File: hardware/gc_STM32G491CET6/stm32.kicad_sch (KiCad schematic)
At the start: 22 parts, among them J7 Conn_02x07_Odd_Even, Y301 16MHz

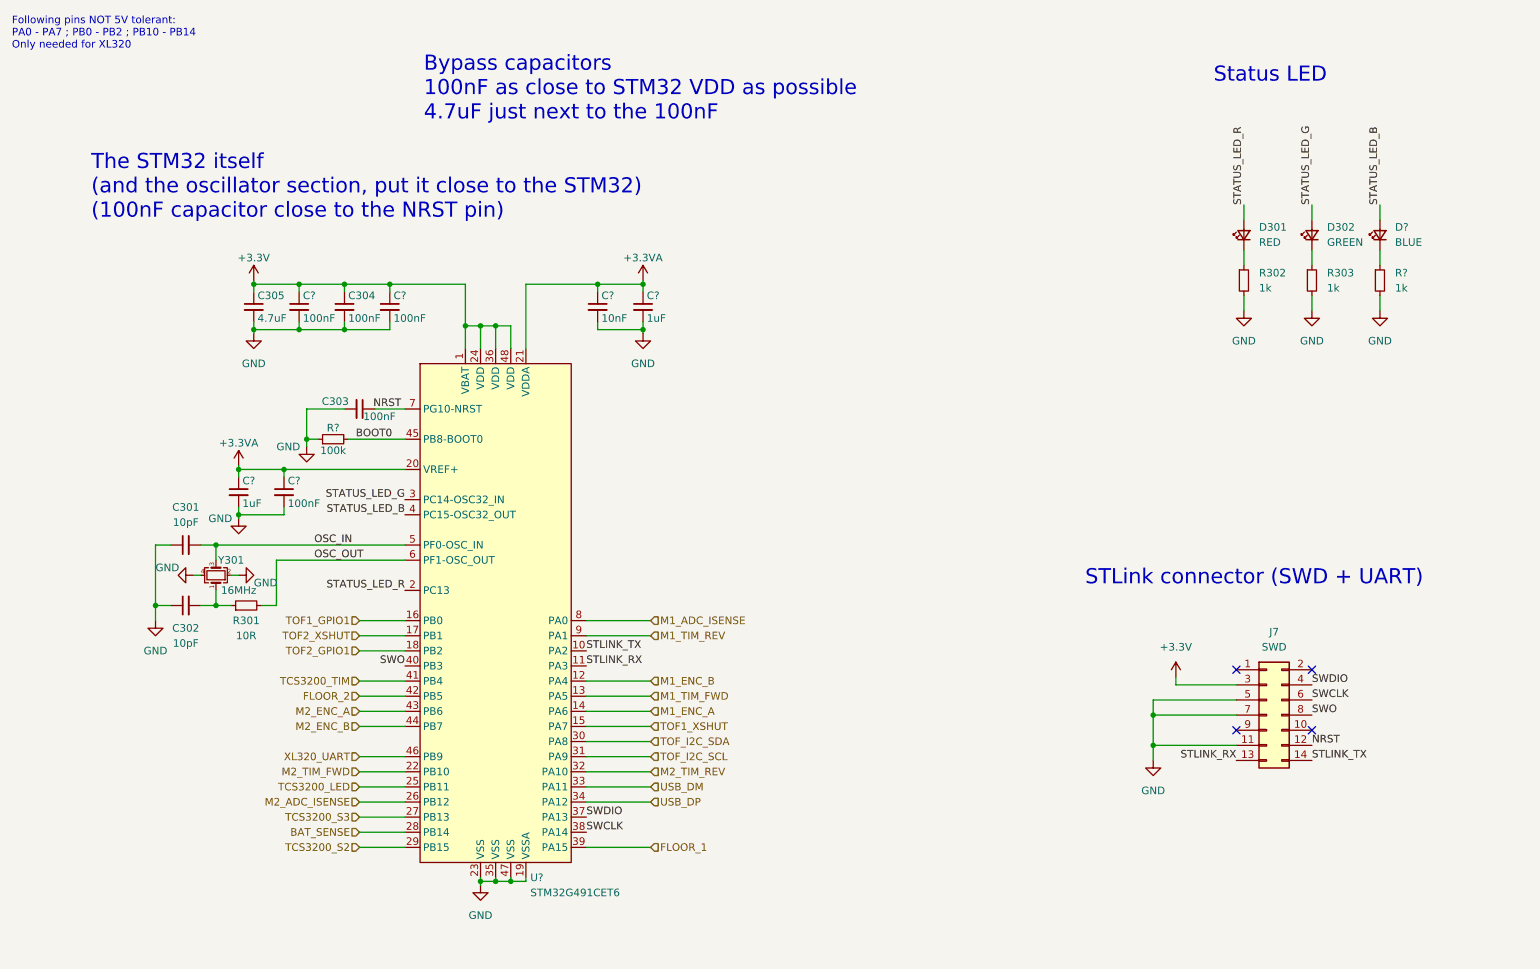
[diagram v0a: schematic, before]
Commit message: Schematics + rough placement
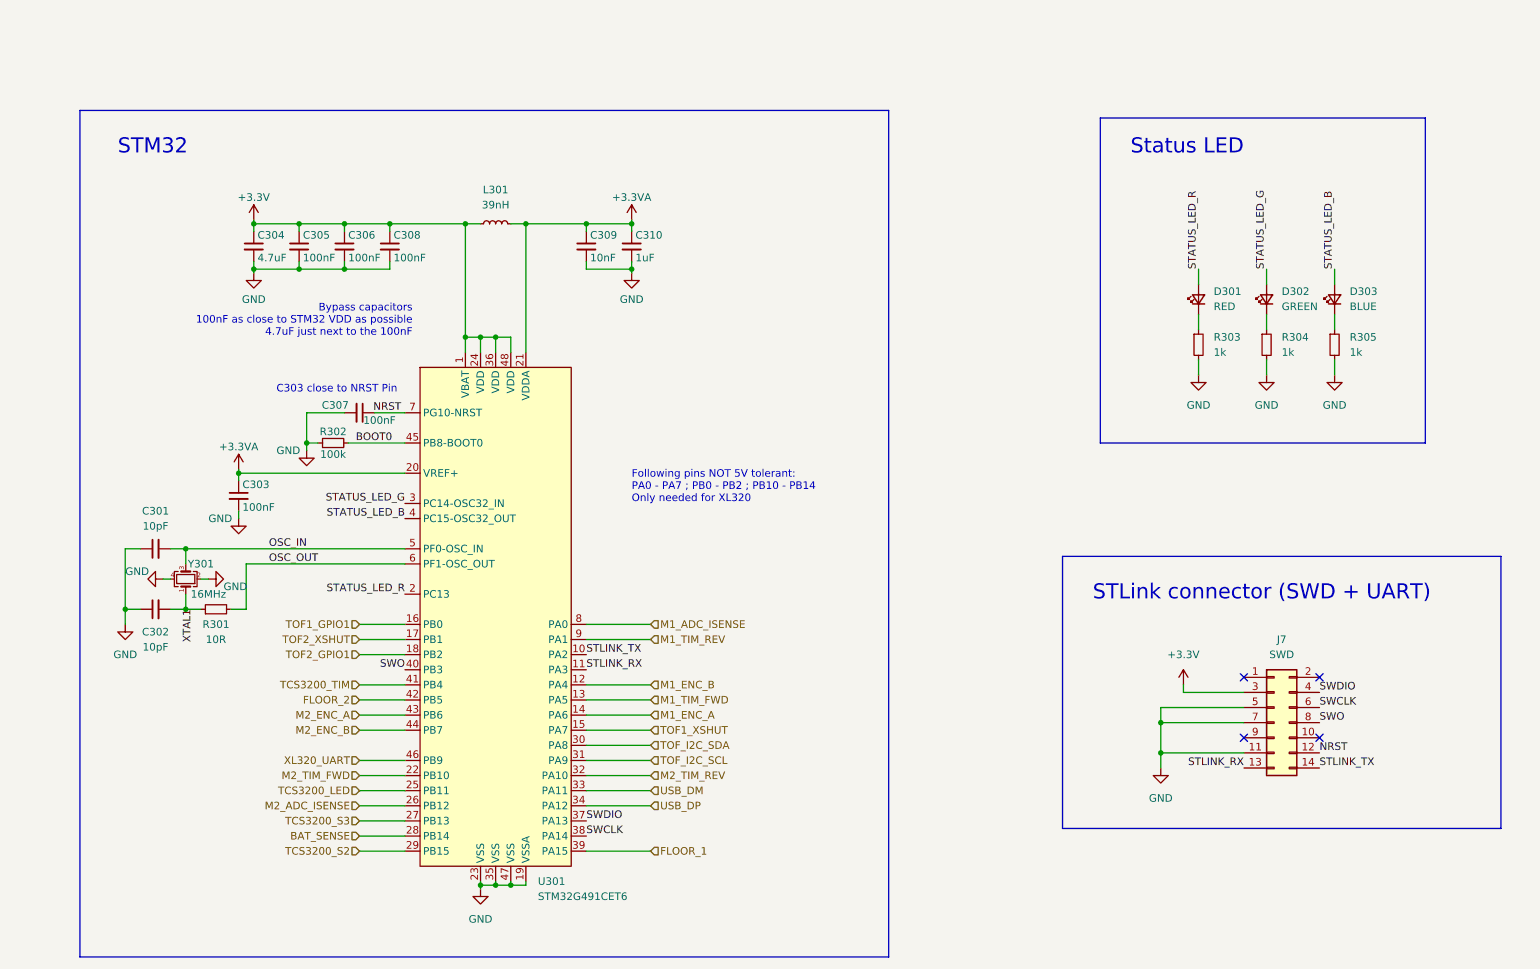
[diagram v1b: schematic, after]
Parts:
- removed C?: 1uF, Capacitor_SMD:C_0603_1608Metric_Pad1.08x0.95mm_HandSolder, symbol Device:C_Small
- removed U?: STM32G491CET6, Package_QFP:LQFP-48_7x7mm_P0.5mm, symbol st:STM32G491CET6
- added L301: 39nH, Inductor_SMD:L_0603_1608Metric, symbol Device:L_Small
- added U301: STM32G491CET6, Package_QFP:LQFP-48_7x7mm_P0.5mm, symbol WITNS_ST:STM32G491CET6
- Y301: footprint Crystal:Crystal_SMD_EuroQuartz_MT-4Pin_3.2x2.5mm_HandSoldering -> Crystal:Crystal_SMD_EuroQuartz_MT-4Pin_3.2x2.5mm
- gave numbers to parts that had none: 8
- renumbered C305 to C304, C304 to C306, C303 to C307, R302 to R303, R303 to R304
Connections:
- net +3.3VA: now also L301.2, U301.20 (VREF+), U301.21 (VDDA)
- net BAT_SENSE: now also U301.28 (PB14)
- net BOOT0: now also U301.45 (PB8-BOOT0)
- net FLOOR_1: now also U301.39 (PA15)
- net FLOOR_2: now also U301.42 (PB5)
- net GND: now also U301.19 (VSSA), U301.23 (VSS), U301.35 (VSS), U301.47 (VSS)
- net M1_ADC_ISENSE: now also U301.8 (PA0)
- net M1_ENC_A: now also U301.14 (PA6)
- net M1_ENC_B: now also U301.12 (PA4)
- net M1_TIM_FWD: now also U301.13 (PA5)
- net M1_TIM_REV: now also U301.9 (PA1)
- net M2_ADC_ISENSE: now also U301.26 (PB12)
- net M2_ENC_A: now also U301.43 (PB6)
- net M2_ENC_B: now also U301.44 (PB7)
- net M2_TIM_FWD: now also U301.22 (PB10)
- net M2_TIM_REV: now also U301.32 (PA10)
- net NRST: now also U301.7 (PG10-NRST)
- net OSC_IN: now also U301.5 (PF0-OSC_IN)
- net OSC_OUT: now also U301.6 (PF1-OSC_OUT)
- net STATUS_LED_B: now also U301.4 (PC15-OSC32_OUT)
- net STATUS_LED_G: now also U301.3 (PC14-OSC32_IN)
- net STATUS_LED_R: now also U301.2 (PC13)
- net STLINK_RX: now also U301.11 (PA3)
- net STLINK_TX: now also U301.10 (PA2)
- net SWCLK: now also U301.38 (PA14)
- net SWDIO: now also U301.37 (PA13)
- net SWO: now also U301.40 (PB3)
- net TCS3200_LED: now also U301.25 (PB11)
- net TCS3200_S2: now also U301.29 (PB15)
- net TCS3200_S3: now also U301.27 (PB13)
- net TCS3200_TIM: now also U301.41 (PB4)
- net TOF1_GPIO1: now also U301.16 (PB0)
- net TOF1_XSHUT: now also U301.15 (PA7)
- net TOF2_GPIO1: now also U301.18 (PB2)
- net TOF2_XSHUT: now also U301.17 (PB1)
- net TOF_I2C_SCL: now also U301.31 (PA9)
- net TOF_I2C_SDA: now also U301.30 (PA8)
- net USB_DM: now also U301.33 (PA11)
- net USB_DP: now also U301.34 (PA12)
- net XL320_UART: now also U301.46 (PB9)
- net XTAL1: now reaches C302.2, R301.1, Y301.1
- net +3V3 renamed +3.3V
- net +3.3V: now also L301.1, U301.1 (VBAT), U301.24 (VDD), U301.36 (VDD), U301.48 (VDD)
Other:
- note added: "C303 close to NRST Pin"
- note added: "STM32"
- note removed: "The STM32 itself (and the oscillator section, put it close to the STM32) (100nF capacitor close to the NRST pin)"
- moved on the sheet: C301, C302, C303, C304, C305, C306, C307, C308, C309, C310, D301, D302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
